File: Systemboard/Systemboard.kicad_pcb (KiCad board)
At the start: 2 copper layers, 175 x 135 mm, 207 parts, among them J1 Conn_01x60, J108 Prog BT, J2 Conn_01x02, J3 Conn_01x01, J4 Conn_01x01, Q1 MMBT5551L, Q2 MMBT5551L, Q3 MMBT5551L, Q4 MMBT5551L, Q5 MMBT5551L, U1 INA226, U10 74HC595, U101 ESP32-WROOM-32E, U103 TLV73333PDBV, U104 PCM2706CPJTR, U11 74HC14, U2 LM358, U201 TLV73333PDBV, U202 PCM5102A, U3 J104D2C12VDC.15S, U301 TLV73333PDBV, U4 J104D2C12VDC.15S, U5 LM2596S-5, U501 TPA3118D2DAPR, U6 LM2596S-3.3, U7 LM2596S-5, U8 LM2596S-ADJ, U9 LTV-817S, Y101 CSTNE12M0G55A000R0

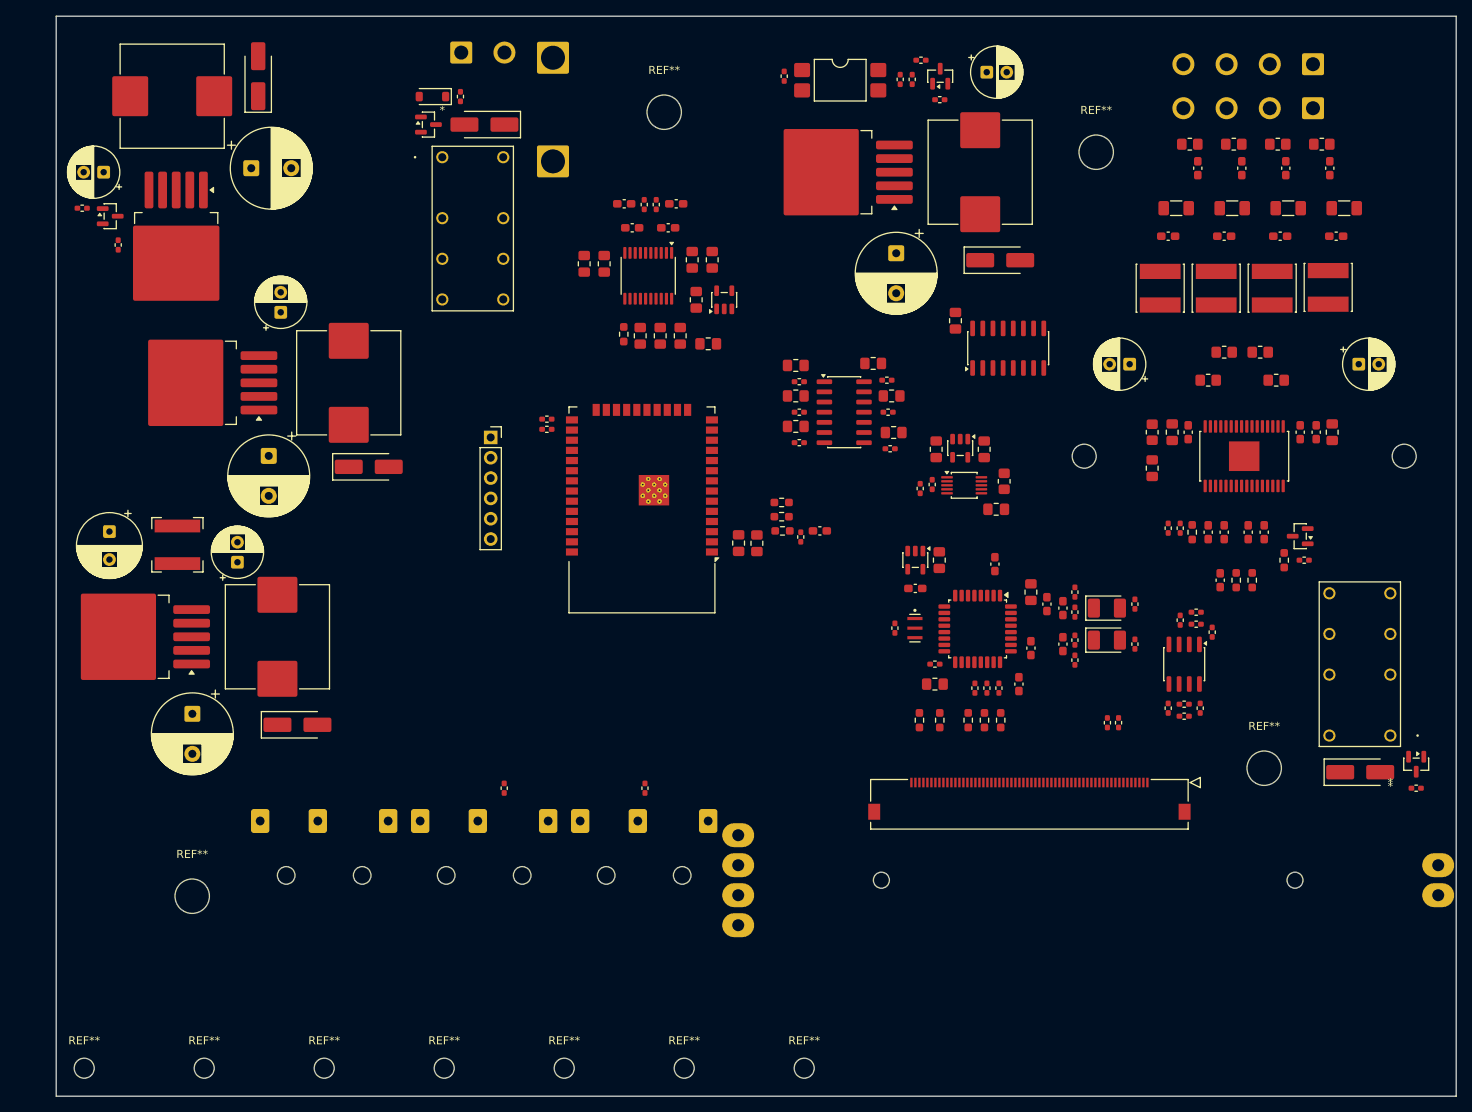
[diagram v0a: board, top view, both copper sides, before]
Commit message: update
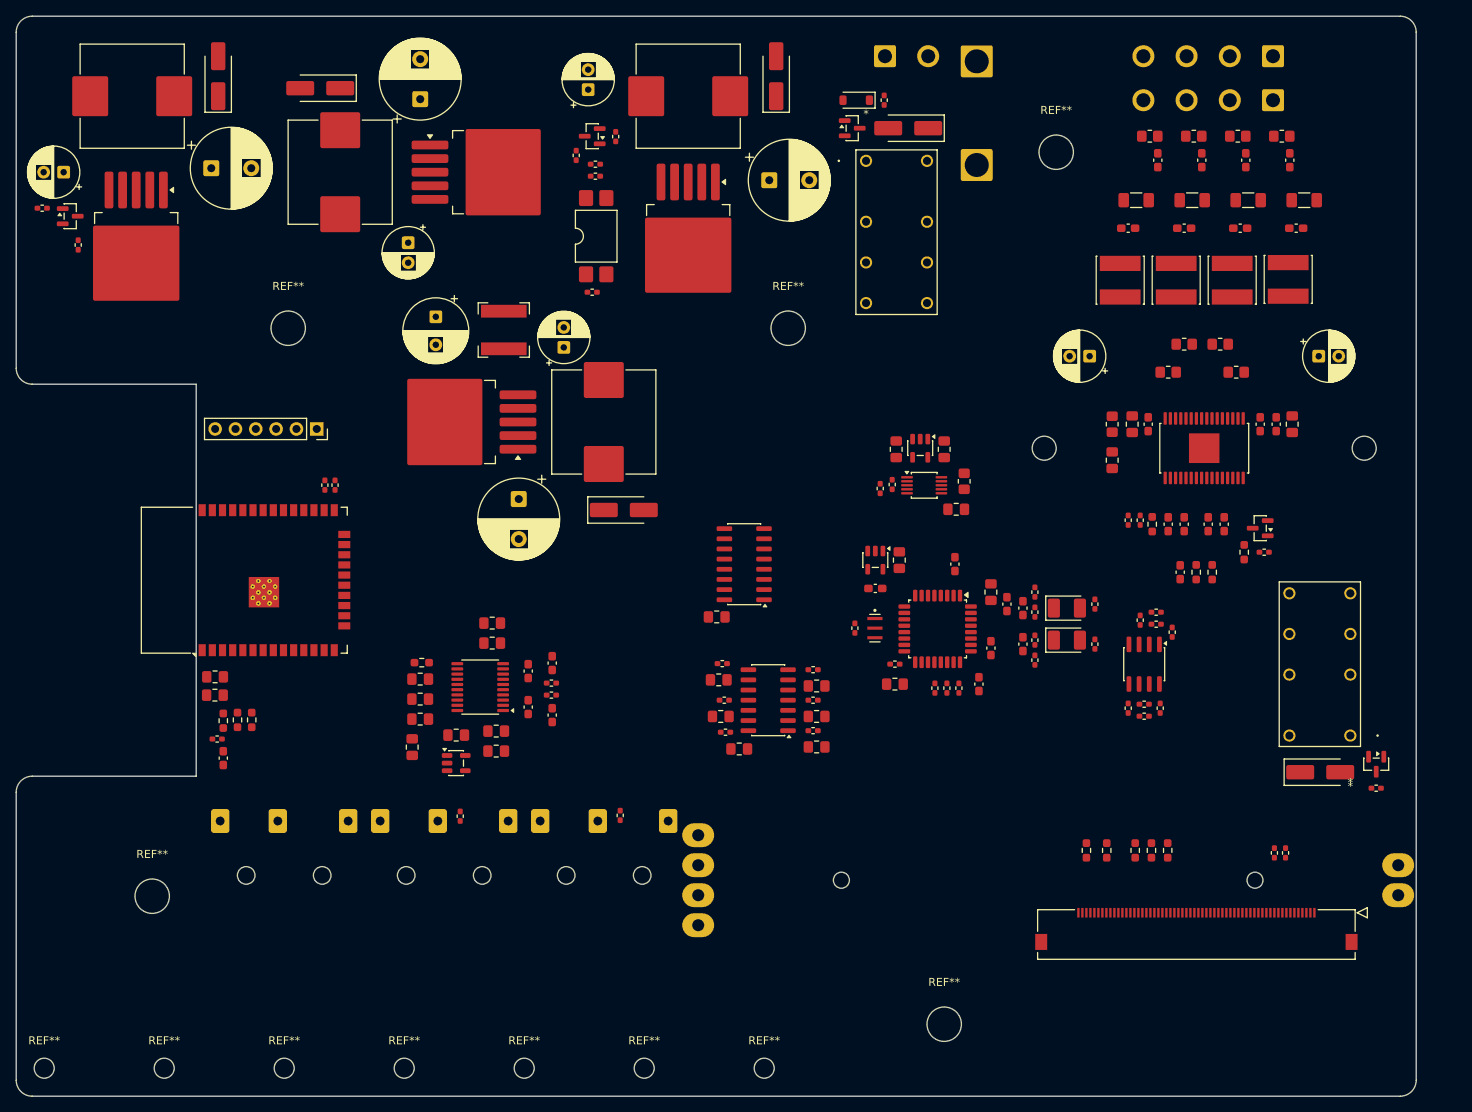
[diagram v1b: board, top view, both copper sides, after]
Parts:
- added REF**: MountingHole_4.3mm_M4, MountingHole:MountingHole_4.3mm_M4, F.Cu at (64.0, 59.0)
- moved C101 79.8 mm to (55.9, 112.7), turned to -90 degrees
- moved R117 77.2 mm to (55.1, 110.4), turned to 180 degrees
- moved R101 73.8 mm to (55.9, 108.1), turned to -90 degrees
- moved R151 72.6 mm to (57.7, 108.0), turned to -90 degrees
- moved R153 71.6 mm to (59.4, 108.0), turned to -90 degrees
- moved C216 70.4 mm to (54.8, 104.9), turned to 180 degrees
- moved C217 67.5 mm to (54.9, 102.6), turned to 0 degrees
- moved C208 67.1 mm to (90.0, 111.9), turned to 180 degrees
- moved U201 66.9 mm to (85.0, 113.4), turned to 0 degrees
- moved C204 65.8 mm to (97.0, 107.4), turned to -90 degrees
- moved C205 63.8 mm to (90.0, 109.4), turned to 180 degrees
- moved R201 62.7 mm to (96.9, 104.9), turned to 0 degrees
- moved C201 62.5 mm to (79.5, 111.4), turned to 90 degrees
- moved C212 62.4 mm to (94.0, 106.4), turned to 90 degrees
- moved C202 62.1 mm to (85.0, 109.9), turned to 180 degrees
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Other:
- outline, holes or cut-outs redrawn
